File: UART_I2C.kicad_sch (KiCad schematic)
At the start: 26 parts, among them J2 Uart1, J3 Uart4, J4 Uart7, J5 Uart(, J6 Uart6, J7 Uart3

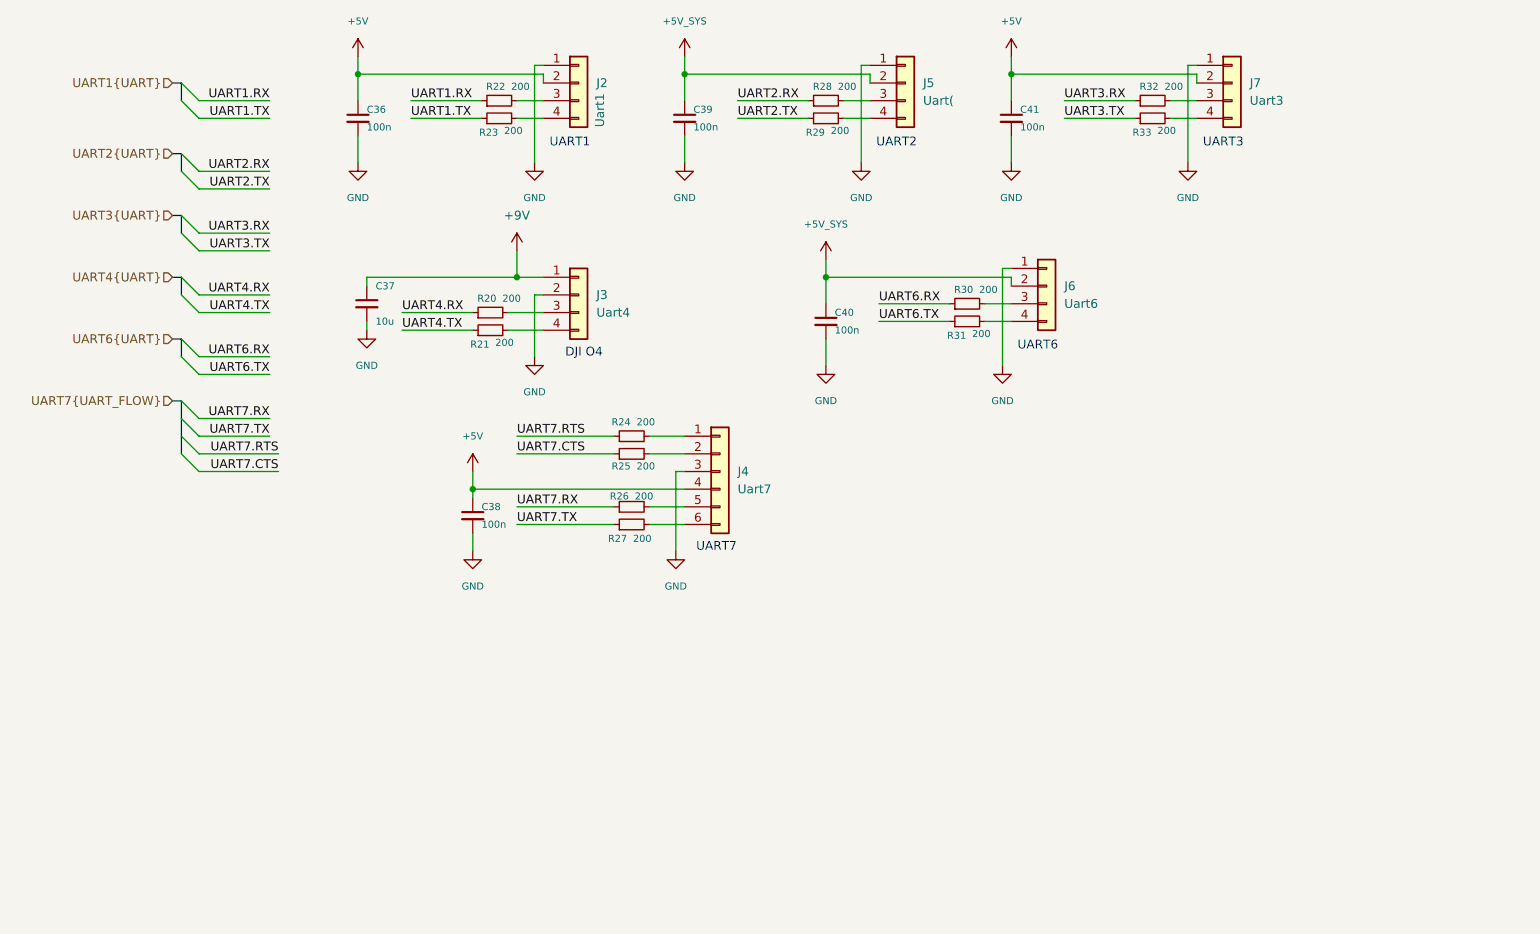
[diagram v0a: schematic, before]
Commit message: update powersupplie
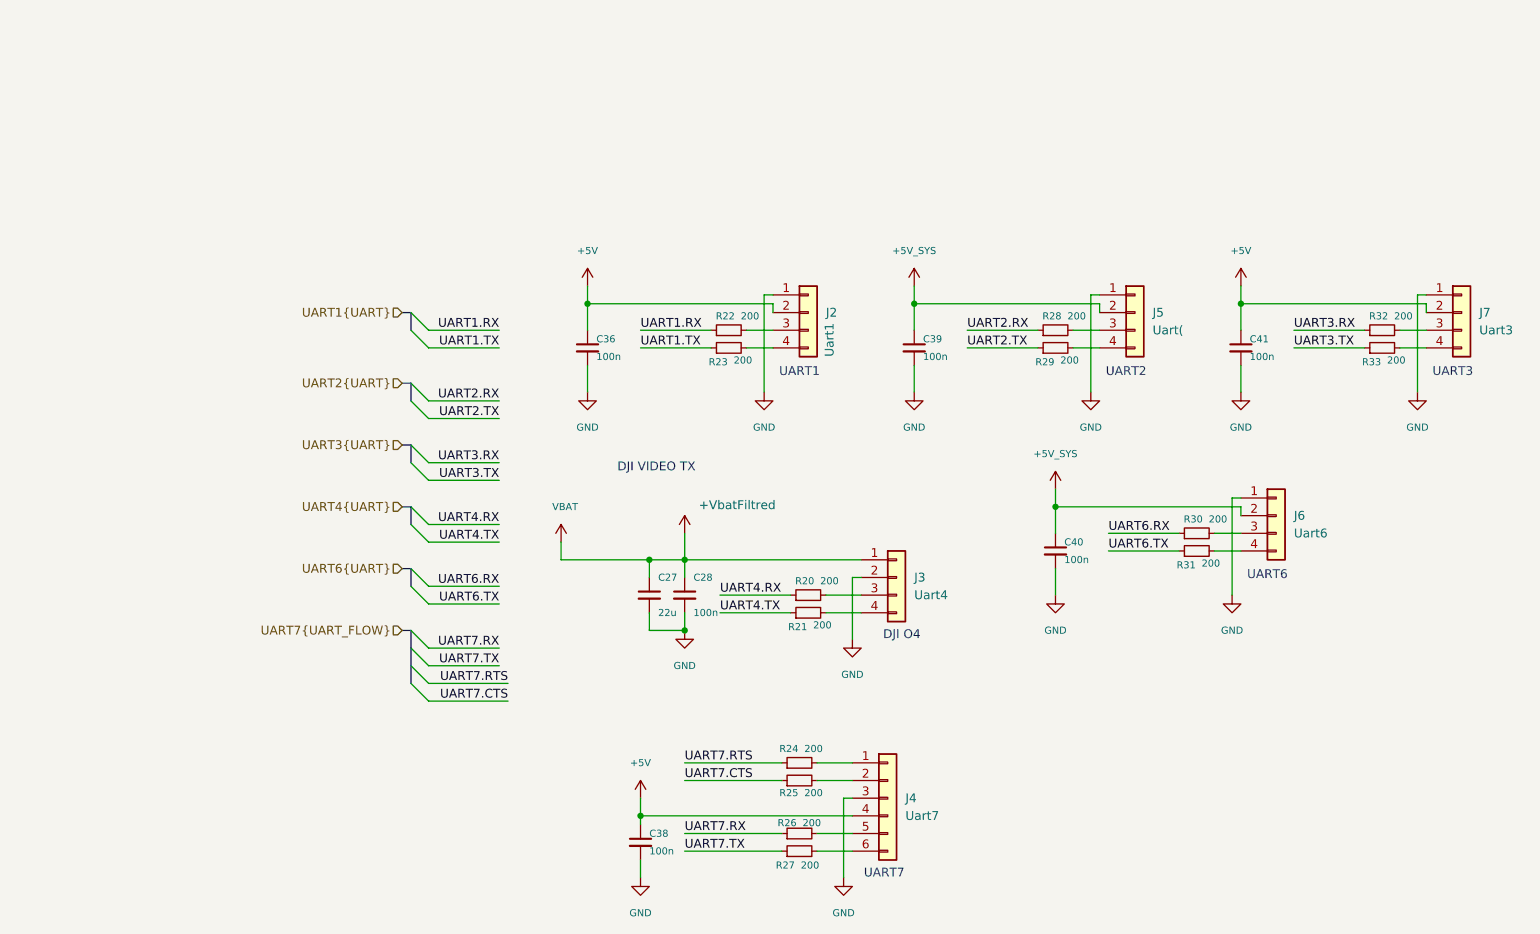
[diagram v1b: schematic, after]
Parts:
- removed C37: 10u, Capacitor_SMD:C_0805_2012Metric, symbol FC01_Project:UART_I2C__C_Small
- added C27: 22u, Capacitor_SMD:C_0805_2012Metric, symbol FC01_Project:POWER__C_Small
- added C28: 100n, Capacitor_SMD:C_0402_1005Metric, symbol FC01_Project:POWER__C_Small
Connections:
- net GND: now also C27.2, C28.2
- net +9V renamed +VbatFiltred
- net +VbatFiltred: now also C27.1, C28.1
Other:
- note added: "DJI VIDEO TX"
- moved on the sheet: C36, C38, C39, C40, C41, J2, J3, J4, J5, J6, J7, R20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
